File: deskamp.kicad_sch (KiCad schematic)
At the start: 0 parts

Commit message: Import ESP32 Mini lib
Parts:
- added U1: mini_esp32, symbol ESP32_mini:mini_esp32
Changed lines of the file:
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@@
 	(generator_version "9.0")
 	(paper "A4")
+	(symbol
+		(lib_id "ESP32_mini:mini_esp32")
+		(at 50.8 38.1 0)
+		(unit 1)
+		(exclude_from_sim no)
+		(in_bom yes)
+		(on_board yes)
+		(dnp no)
+		(fields_autoplaced yes)
+		(property "Reference" "U1"
+			(at 51.435 34.29 0)
+			(effects
+				(font
+					(size 1.27 1.27)
+				)
+			)
+		)
+		(property "Value" "mini_esp32"
+			(at 51.435 36.83 0)
+			(effects
+				(font
+					(size 1.27 1.27)
+				)
+			)
+		)
+		(property "Footprint" ""
+			(at 54.61 35.56 0)
+			(effects
+				(font
+					(size 1.27 1.27)
+				)
+				(hide yes)
+			)
+		)
+		(property "Datasheet" ""
+			(at 54.61 35.56 0)
+			(effects
+				(font
+					(size 1.27 1.27)
+				)
+				(hide yes)
+			)
+		)
+		(property "Description" ""
+			(at 50.8 38.1 0)
+			(effects
+				(font
+					(size 1.27 1.27)
+				)
+				(hide yes)
+			)
+		)
+		(pin "4"
+		)
+		(pin "5"
+		)
+		(pin "1"
+		)
+		(pin "2"
+		)
+		(pin "3"
+		)
+		(pin "34"
+		)
+		(pin "36"
+		)
+		(pin "32"
+		)
+		(pin "18"
+		)
+		(pin "13"
+		)
+		(pin "31"
+		)
+		(pin "29"
+		)
+		(pin "8"
+		)
+		(pin "20"
+		)
+		(pin "30"
+		)
+		(pin "10"
+		)
+		(pin "28"
+		)
+		(pin "9"
+		)
+		(pin "11"
+		)
+		(pin "7"
+		)
+		(pin "27"
+		)
+		(pin "25"
+		)
+		(pin "12"
+		)
+		(pin "26"
+		)
+		(pin "6"
+		)
+		(pin "24"
+		)
+		(pin "35"
+		)
+		(pin "16"
+		)
+		(pin "33"
+		)
+		(pin "22"
+		)
+		(pin "15"
+		)
+		(pin "19"
+		)
+		(pin "21"
+		)
+		(pin "23"
+		)
+		(pin "40"
+		)
+		(pin "39"
+		)
+		(pin "38"
+		)
+		(pin "37"
+		)
+		(pin "14"
+		)
+		(pin "17"
+		)
+		(instances
+			(project ""
+				(path "/59ddc706-9eaa-4fe8-a820-1bc51705c457"
+					(reference "U1")
+					(unit 1)
+				)
+			)
+		)
+	)
 	(sheet_instances
 		(path "/"

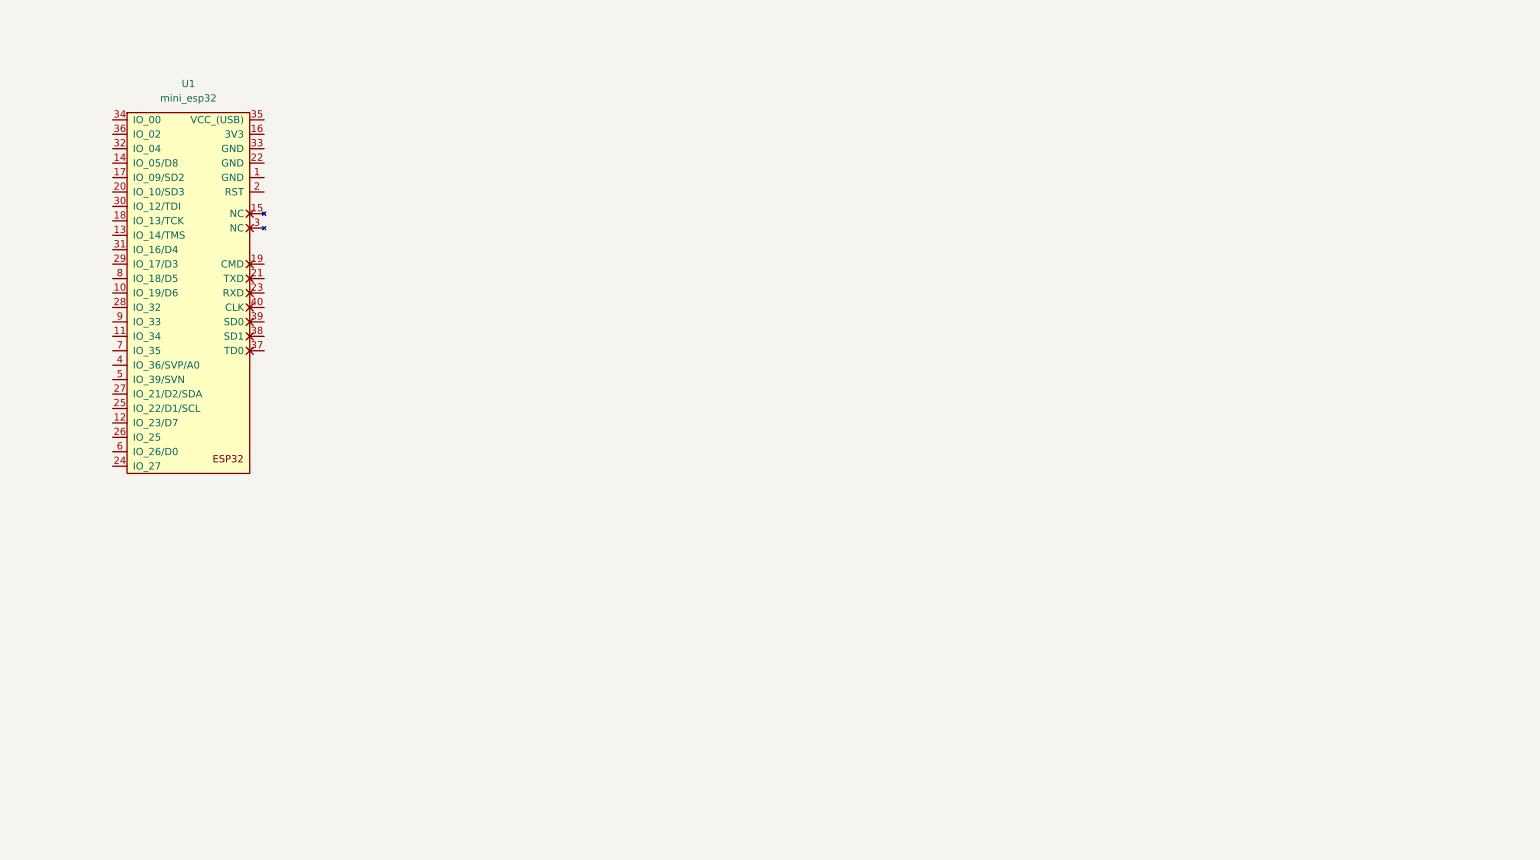
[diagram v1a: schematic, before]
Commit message: Start building switch logic
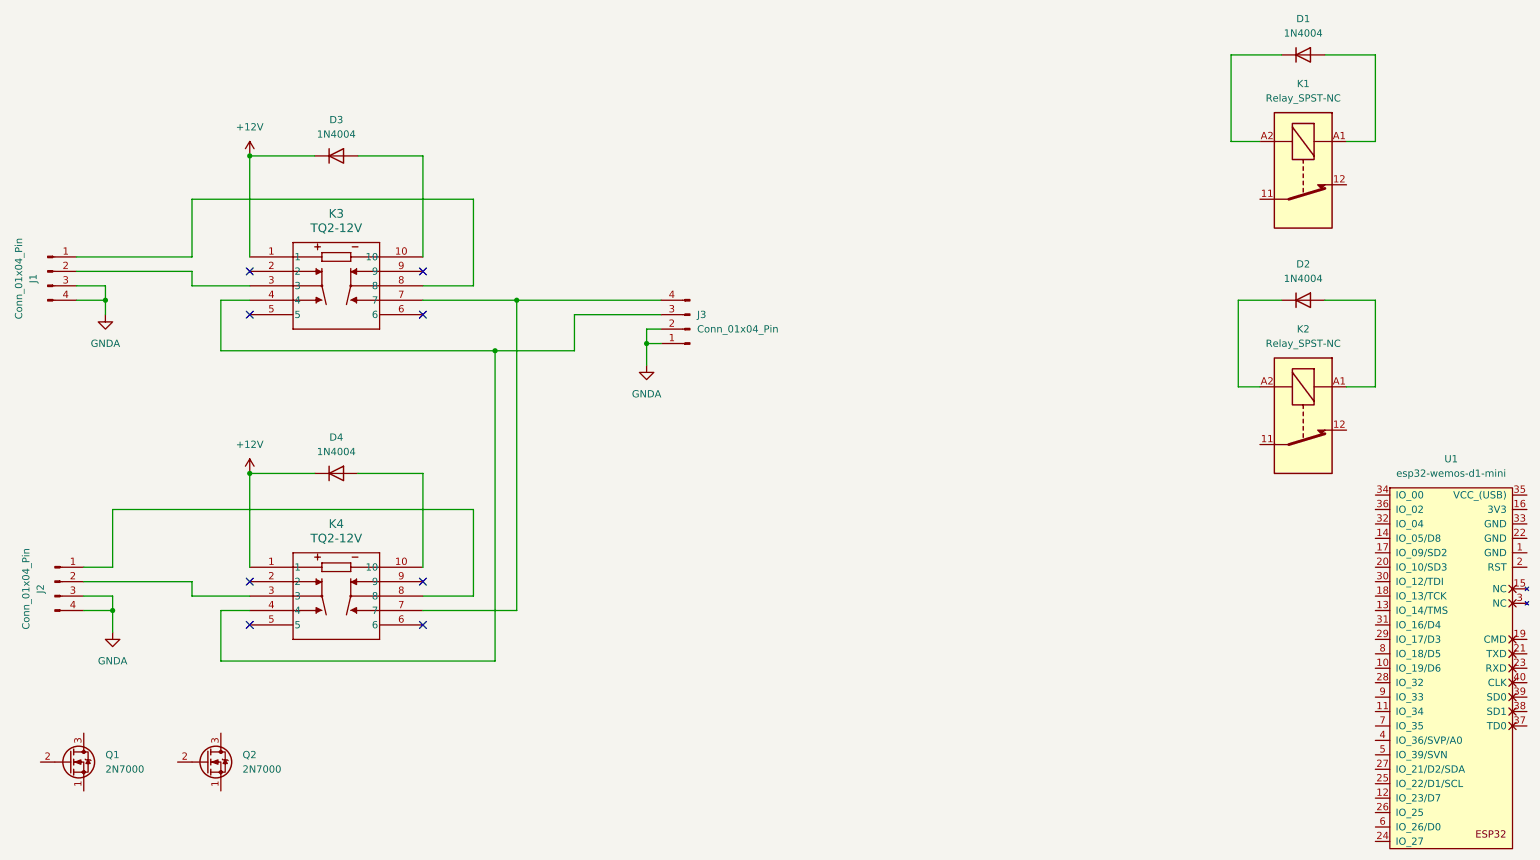
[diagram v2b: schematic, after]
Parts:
- removed U1: mini_esp32, symbol ESP32_mini:mini_esp32
- added D1, D2, D3, D4: 1N4004, Diode_THT:D_DO-41_SOD81_P10.16mm_Horizontal, symbol Diode:1N4004
- added J1, J2, J3: Conn_01x04_Pin, Connector_JST:JST_XH_B4B-XH-AM_1x04_P2.50mm_Vertical, symbol Connector:Conn_01x04_Pin
- added K1, K2: Relay_SPST-NC, symbol Relay:Relay_SPST-NC
- added K3, K4: TQ2-12V, RELAY_TQ2_PAN, symbol 2025-10-05_02-56-43:TQ2-12V
- added Q1, Q2: 2N7000, Package_TO_SOT_THT:TO-92L_HandSolder, symbol Transistor_FET:2N7000
- added U1: esp32-wemos-d1-mini, esp32-wemos-d1-mini:esp32-wemos-d1-mini, symbol esp32-wemos-d1-mini:esp32-wemos-d1-mini
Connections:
- new net: D2.2 (A), K2.A1
- new net: D2.1 (K), K2.A2
- new net: J2.1 (Pin_1), K4.8
- new net: J2.2 (Pin_2), K4.3
- new net: J1.1 (Pin_1), K3.8
- new net: J1.2 (Pin_2), K3.3
- new net: D4.2 (A), K4.10
- new net: D1.2 (A), K1.A1
- new net: D1.1 (K), K1.A2
- new net: D3.2 (A), K3.10
- new net: J3.3 (Pin_3), K3.4, K4.4
- new net: J3.4 (Pin_4), K3.7, K4.7
- new net +12V: D3.1 (K), D4.1 (K), K3.1, K4.1
- new net GNDA: J1.3 (Pin_3), J1.4 (Pin_4), J2.3 (Pin_3), J2.4 (Pin_4), J3.1 (Pin_1), J3.2 (Pin_2)
- no-connect marks 0 -> 8
